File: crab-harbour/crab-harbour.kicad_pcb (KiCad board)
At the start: 2 copper layers, 110.7 x 69.7 mm, 38 parts, among them J1 MJ-4PP-9, SW10 SW_PUSH, SW11 SW_PUSH, SW12 SW_PUSH, SW14 SW_PUSH, SW15 SW_PUSH, SW16 SW_PUSH, SW17 SW_PUSH, SW18 SW_PUSH, SW19 SW_PUSH, SW2 SW_PUSH, SW20 SW_PUSH, SW3 SW_PUSH, SW4 SW_PUSH, SW5 SW_PUSH, SW6 SW_PUSH, SW8 SW_PUSH, SW9 SW_PUSH, U1 ProMicro

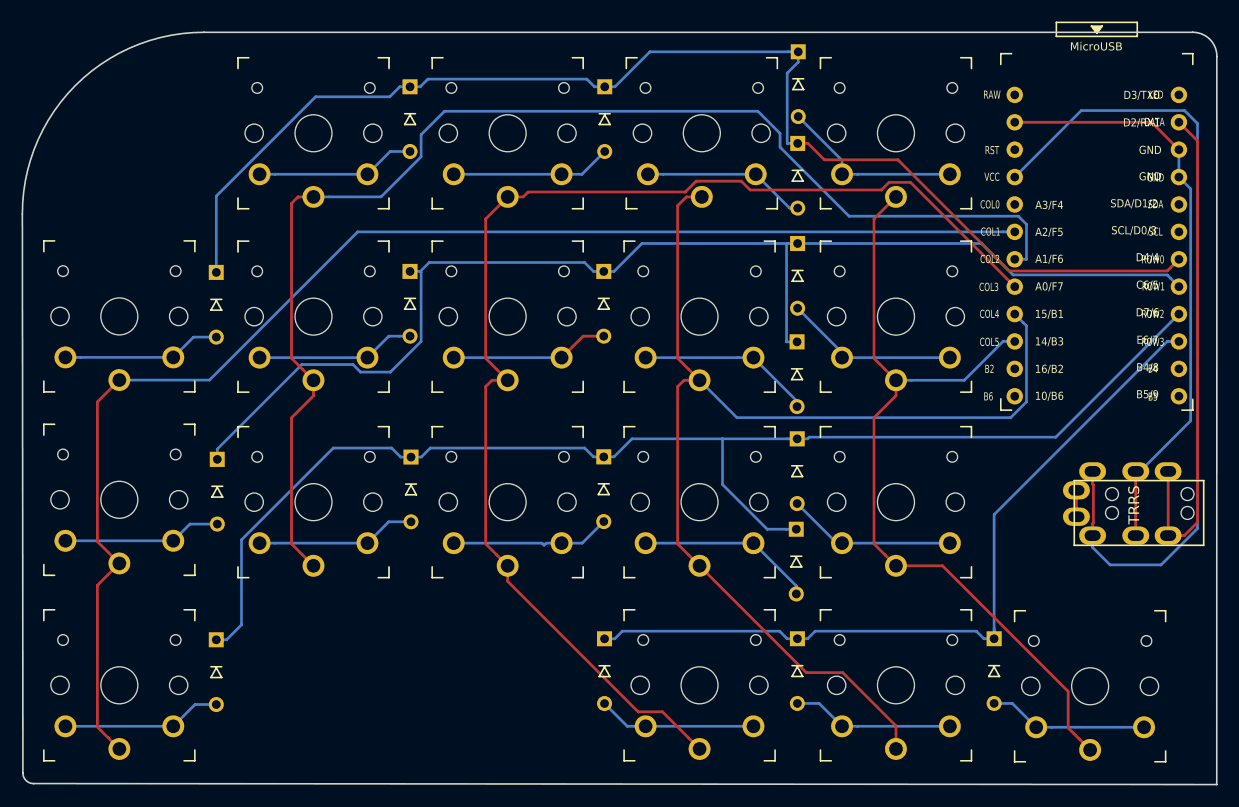
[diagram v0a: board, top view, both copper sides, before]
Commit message: Add files via upload
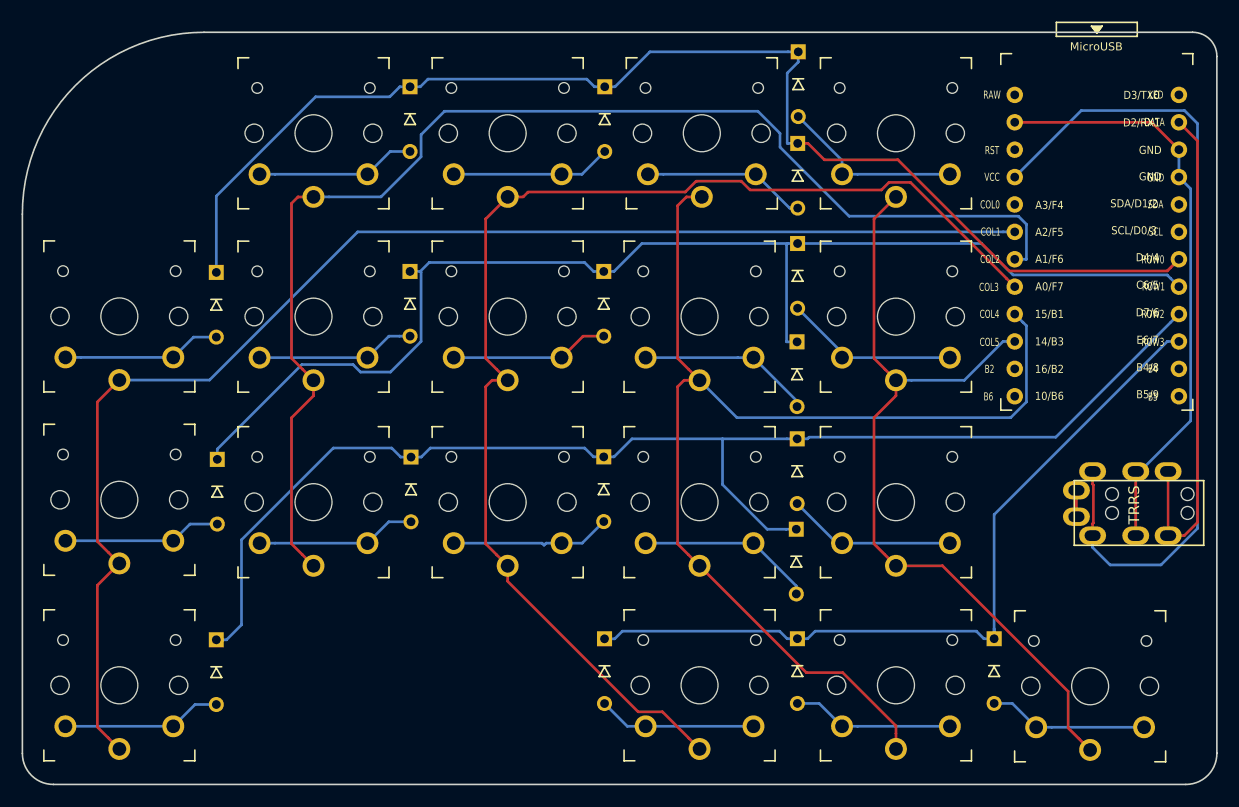
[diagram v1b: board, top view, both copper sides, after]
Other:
- outline, holes or cut-outs redrawn
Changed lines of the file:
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@@
   (general
     (thickness 1.6)
-    (drawings 7)
+    (drawings 8)
     (tracks 285)
     (zones 0)
@@
     (visible_elements FFFFEFFF)
     (pcbplotparams
-      (layerselection 0x010f0_ffffffff)
+      (layerselection 0x010c0_ffffffff)
       (usegerberextensions true)
       (usegerberattributes false)
@@
     )
   )
+  (gr_arc (start 37.876821 87.983263) (end 35.009924 87.97) (angle -90.52693434) (layer Edge.Cuts) (width 0.15))
+  (gr_arc (start 142.883294 87.983067) (end 142.87 90.849964) (angle -90.92679038) (layer Edge.Cuts) (width 0.15))
   (gr_arc (start 143.531624 23.340059) (end 145.751623 23.360058) (angle -91.07419804) (layer Edge.Cuts) (width 0.15))
-  (gr_arc (start 36.04 89.79) (end 35.06 89.79) (angle -91.15733307) (layer Edge.Cuts) (width 0.15))
   (gr_arc (start 51.819952 37.930001) (end 51.85 21.12) (angle -90.23866858) (layer Edge.Cuts) (width 0.15))
   (gr_line (start 143.510001 21.120075) (end 51.85 21.12) (angle 90) (layer Edge.Cuts) (width 0.15))
-  (gr_line (start 35.009924 37.969976) (end 35.06 89.79) (angle 90) (layer Edge.Cuts) (width 0.15))
-  (gr_line (start 36.059794 90.7698) (end 145.74 90.86) (angle 90) (layer Edge.Cuts) (width 0.15))
-  (gr_line (start 145.75 23.36) (end 145.74 90.86) (angle 90) (layer Edge.Cuts) (width 0.15))
+  (gr_line (start 35.009924 37.969976) (end 35.009924 87.97) (angle 90) (layer Edge.Cuts) (width 0.15))
+  (gr_line (start 37.89 90.85) (end 142.87 90.849964) (angle 90) (layer Edge.Cuts) (width 0.15))
+  (gr_line (start 145.75 23.36) (end 145.75 87.949988) (angle 90) (layer Edge.Cuts) (width 0.15))
   (segment (start 70.0015 26.17) (end 70.95 26.17) (width 0.25) (layer B.Cu) (net 1))
   (segment (start 69.071199 27.100301) (end 70.0015 26.17) (width 0.25) (layer B.Cu) (net 1))
